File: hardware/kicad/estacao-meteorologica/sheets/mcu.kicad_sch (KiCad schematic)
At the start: 1 part, among them U5 NUCLEO-F446RE

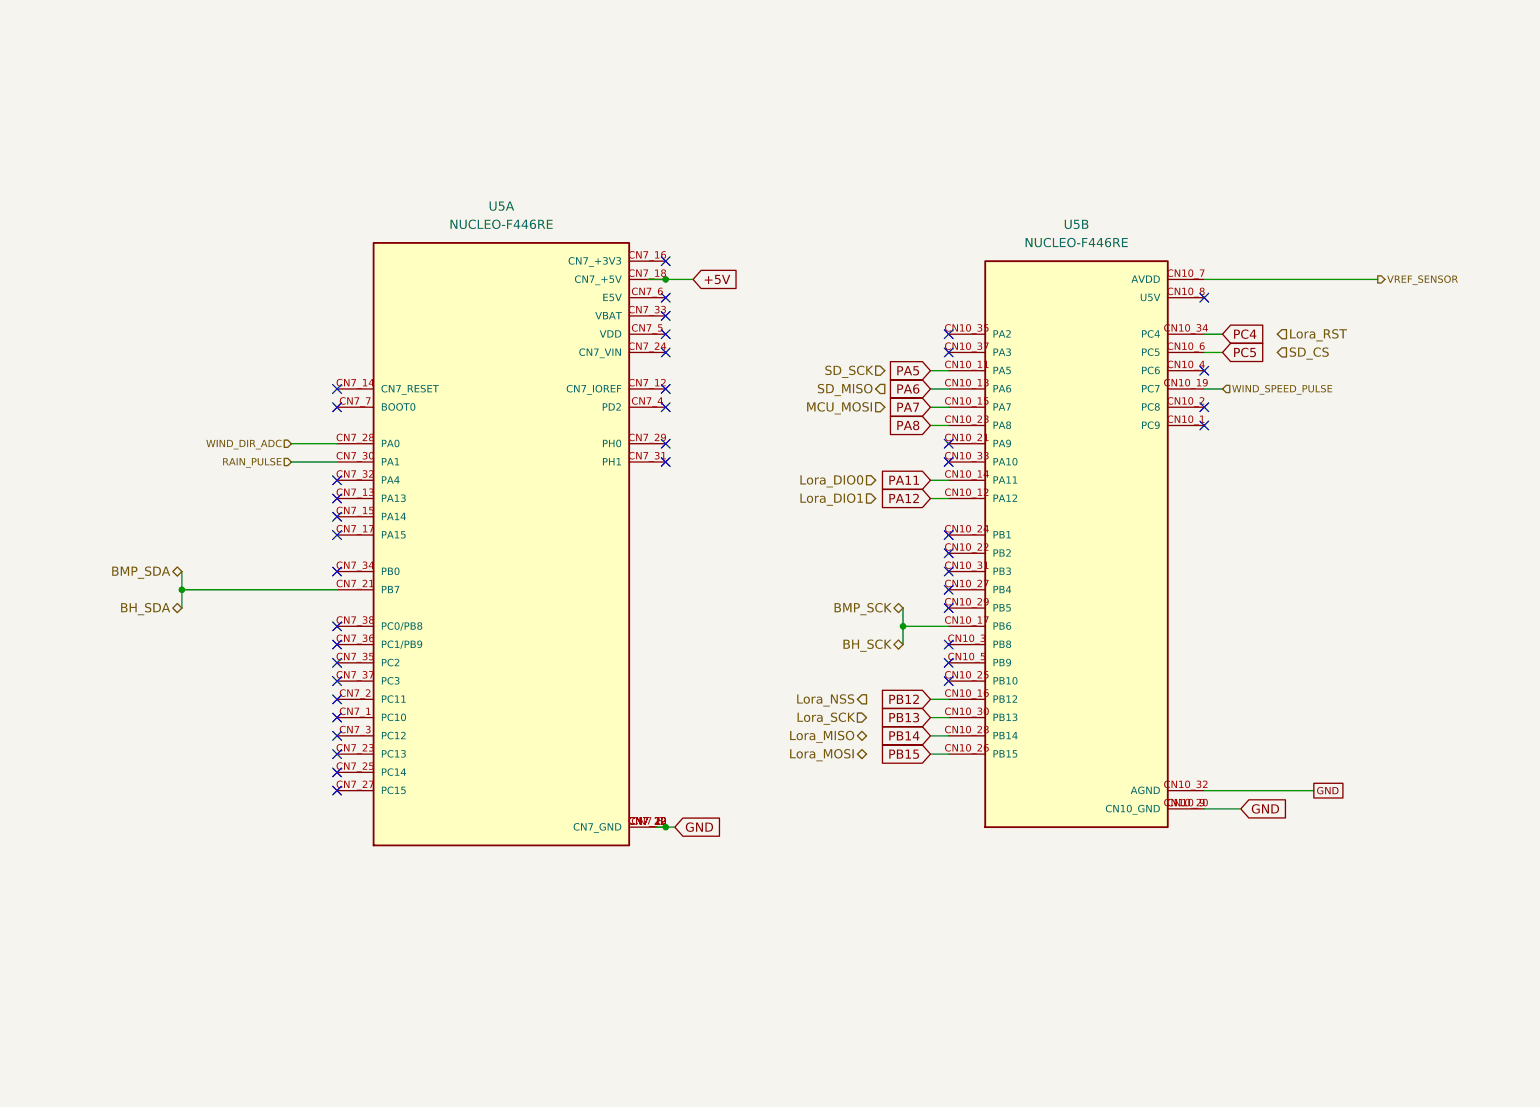
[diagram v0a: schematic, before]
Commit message: refatoracao: atualizacoes de hardware e falta revisao LoRa
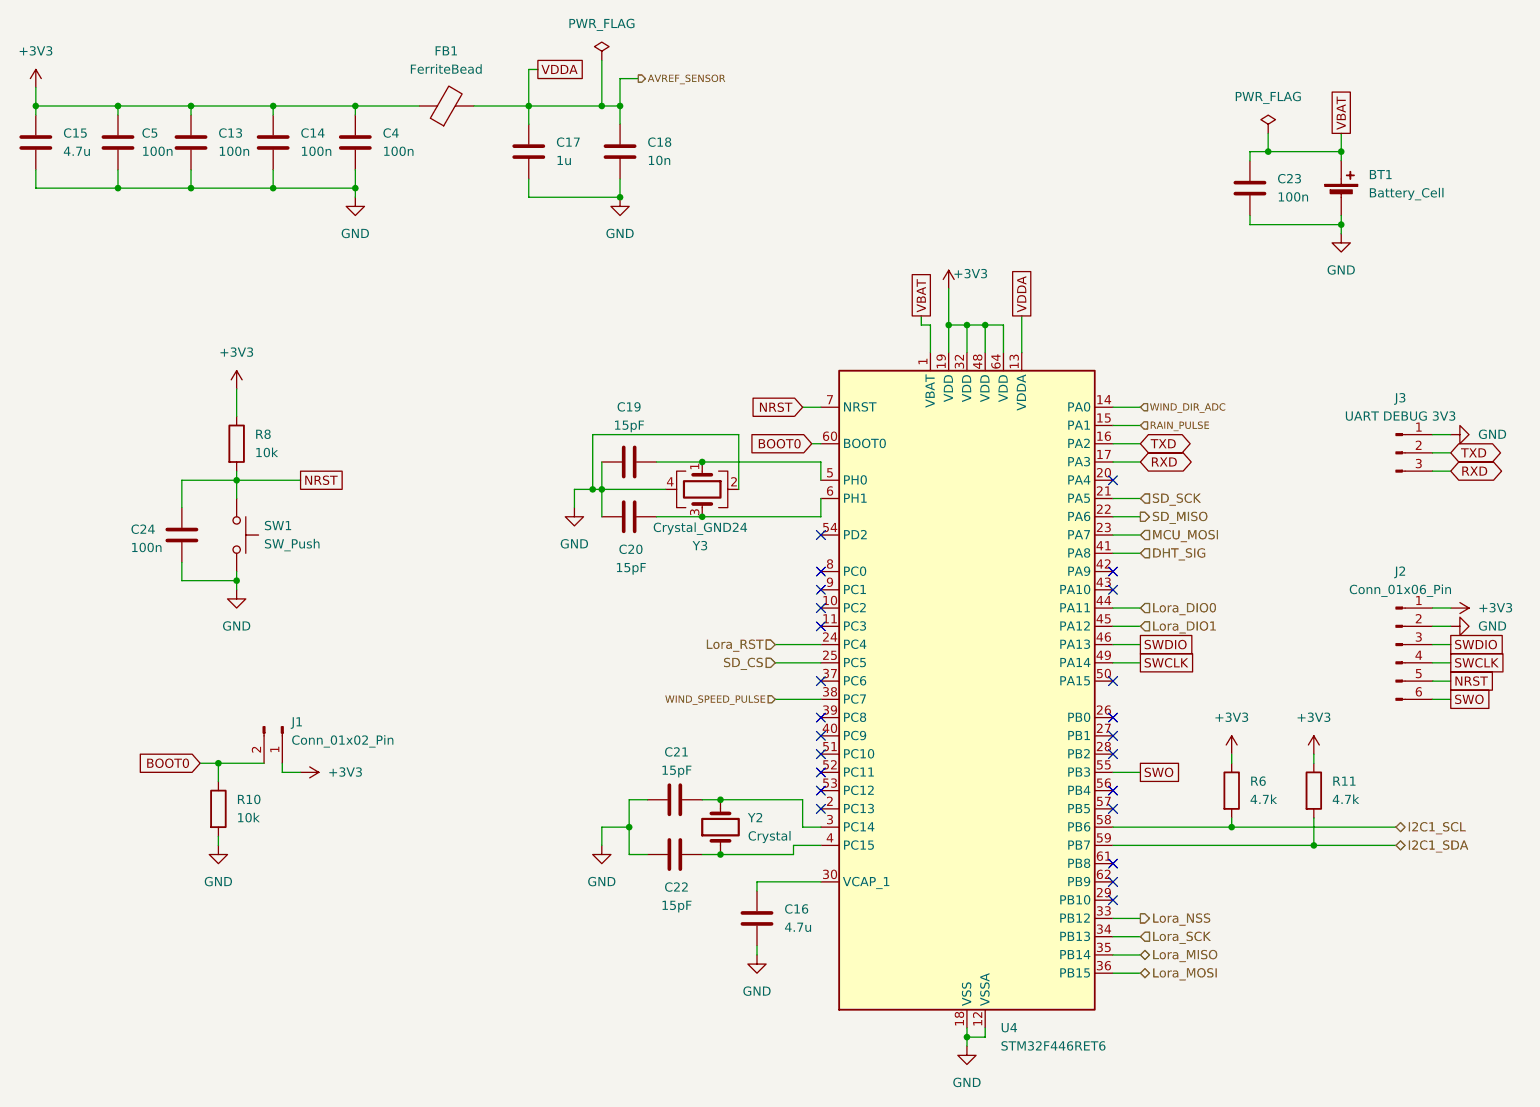
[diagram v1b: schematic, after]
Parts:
- removed U5: NUCLEO-F446RE, myLibrary:MODULE_NUCLEO-F446RE, symbol Hardware_MCU:NUCLEO-F446RE_Morpho
- added BT1: Battery_Cell, symbol Device:Battery_Cell
- added C13, C14, C23, C24, C4, C5: 100n, symbol Device:C
- added C15, C16: 4.7u, symbol Device:C
- added C17: 1u, symbol Device:C
- added C18: 10n, symbol Device:C
- added C19, C20, C21, C22: 15pF, symbol Device:C
- added FB1: FerriteBead, symbol Device:FerriteBead
- added J1: Conn_01x02_Pin, symbol Connector:Conn_01x02_Pin
- added J2: Conn_01x06_Pin, symbol Connector:Conn_01x06_Pin
- added J3: UART DEBUG 3V3, symbol Connector:Conn_01x03_Pin
- added R10, R8: 10k, symbol Device:R
- added R11, R6: 4.7k, symbol Device:R
- added SW1: SW_Push, symbol Switch:SW_Push
- added U4: STM32F446RET6, Package_QFP:LQFP-64_10x10mm_P0.5mm, symbol MCU_ST_STM32F4:STM32F446RETx
- added Y2: Crystal, symbol Device:Crystal
- added Y3: Crystal_GND24, symbol Device:Crystal_GND24
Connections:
- net GND: now also BT1.2 (-), C13.2, C14.2, C15.2, C16.2, C17.2, C18.2, C19.1, C20.1, C21.1, C22.1, C23.2, C24.2, C4.2, C5.2, J2.2 (Pin_2), J3.1 (Pin_1), R10.2, SW1.2, U4.12 (VSSA), U4.18 (VSS), U4.31 (VSS), U4.47 (VSS), U4.63 (VSS), Y3.2, Y3.4
- net Lora_DIO0: now also U4.44 (PA11)
- net Lora_DIO1: now also U4.45 (PA12)
- net Lora_MISO: now also U4.35 (PB14)
- net Lora_MOSI: now also U4.36 (PB15)
- net Lora_NSS: now also U4.33 (PB12)
- net Lora_RST: now also U4.24 (PC4)
- net Lora_SCK: now also U4.34 (PB13)
- net MCU_MOSI: now also U4.23 (PA7)
- net RAIN_PULSE: now also U4.15 (PA1)
- net SD_CS: now also U4.25 (PC5)
- net SD_MISO: now also U4.22 (PA6)
- net SD_SCK: now also U4.21 (PA5)
- net WIND_DIR_ADC: now also U4.14 (PA0)
- net WIND_SPEED_PULSE: now also U4.38 (PC7)
- new net: C22.2, U4.4 (PC15), Y2.1
- new net: C21.2, U4.3 (PC14), Y2.2
- new net: C19.2, U4.5 (PH0), Y3.1
- new net: C20.2, U4.6 (PH1), Y3.3
- new net: C16.1, U4.30 (VCAP_1)
- new net +3V3: C13.1, C14.1, C15.1, C4.1, C5.1, FB1.1, J1.1 (Pin_1), J2.1 (Pin_1), R11.1, R6.1, R8.1, U4.19 (VDD), U4.32 (VDD), U4.48 (VDD), U4.64 (VDD)
- new net BOOT0: J1.2 (Pin_2), R10.1, U4.60 (BOOT0)
- new net DHT_SIG: U4.41 (PA8)
- new net I2C1_SCL: R6.2, U4.58 (PB6)
- new net I2C1_SDA: R11.2, U4.59 (PB7)
- new net NRST: C24.1, J2.5 (Pin_5), R8.2, SW1.1, U4.7 (NRST)
- new net RXD: J3.3 (Pin_3), U4.17 (PA3)
- new net SWCLK: J2.4 (Pin_4), U4.49 (PA14)
- new net SWDIO: J2.3 (Pin_3), U4.46 (PA13)
- new net SWO: J2.6 (Pin_6), U4.55 (PB3)
- new net TXD: J3.2 (Pin_2), U4.16 (PA2)
- new net VBAT: BT1.1 (+), C23.1, U4.1 (VBAT)
- new net VDDA: C17.1, C18.1, FB1.2, U4.13 (VDDA)
- no-connect marks 42 -> 24
